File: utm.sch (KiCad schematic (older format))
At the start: 9 parts

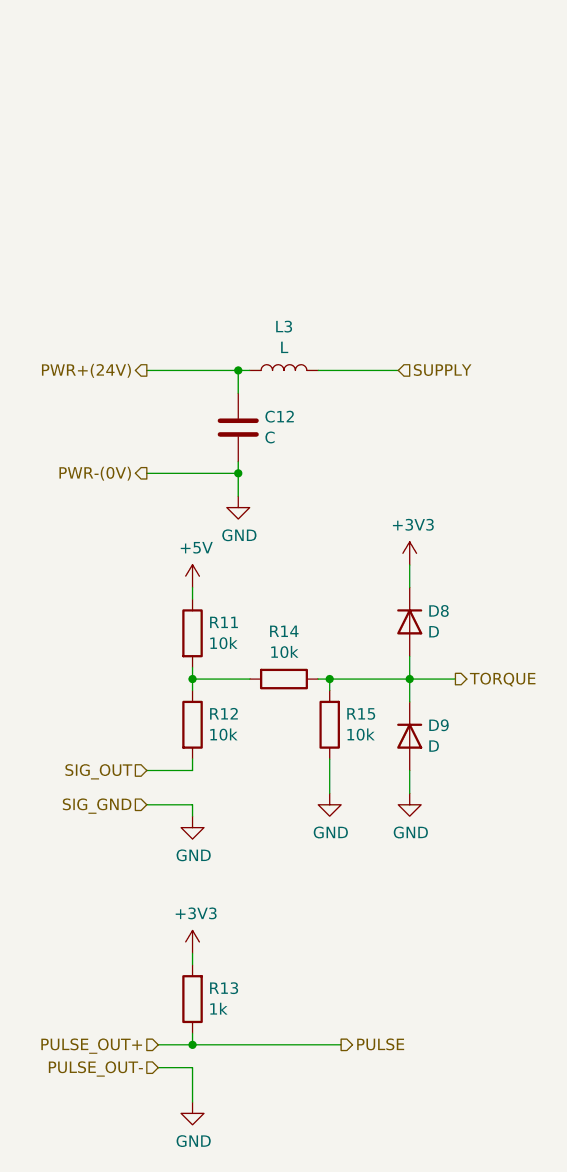
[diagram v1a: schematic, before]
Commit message: 設計修正
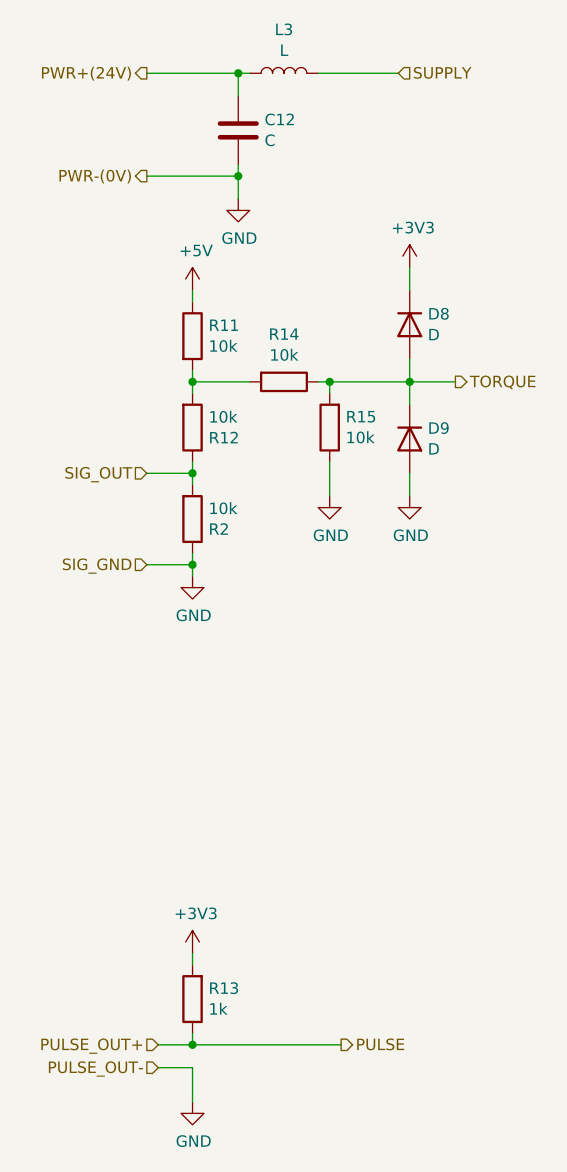
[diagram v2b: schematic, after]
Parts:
- added R2: 10k, Resistor_SMD:R_0603_1608Metric, symbol Device:R
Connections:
- net GND: now also R2.1
- net SIG_OUT: now also R12.1, R2.2; no longer R12.2
- net at R11.2, R14.2: now also R12.2; no longer R12.1
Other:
- moved on the sheet: C12, D8, D9, L3, R11, R12, R14, R15
